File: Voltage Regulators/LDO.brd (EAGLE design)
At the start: 16.8 x 13.3 mm, 4 parts

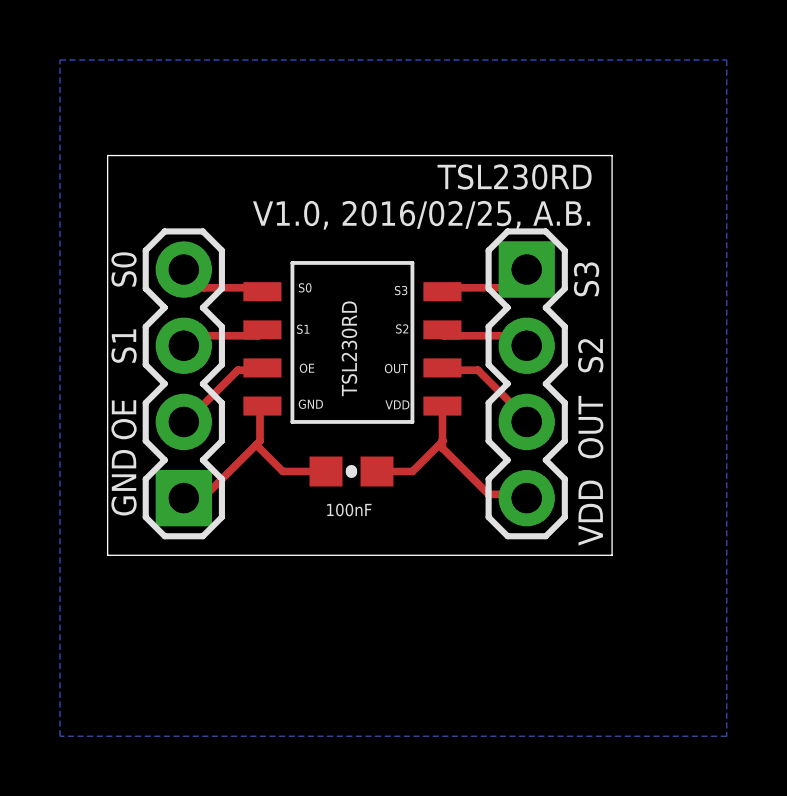
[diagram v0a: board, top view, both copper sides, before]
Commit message: new boards
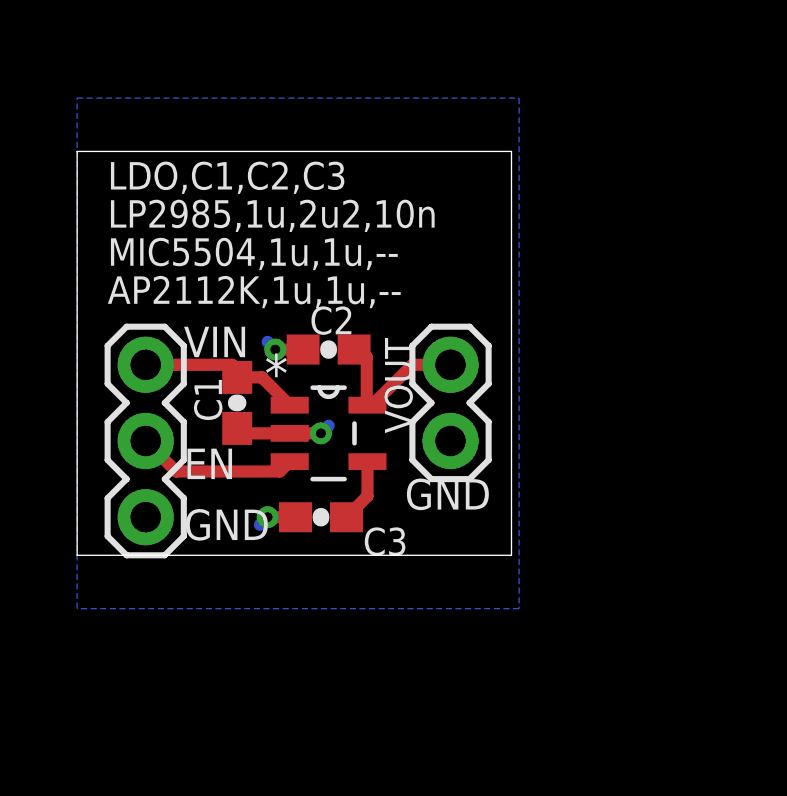
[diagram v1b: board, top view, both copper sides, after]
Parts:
- removed 100NF: 100nF, SparkFun-Capacitors:0603-CAP
- removed J1, J2: (no value), SparkFun-Connectors:1X04
- removed U$1: TSL230RDSMD, awqua_eagle_library:TSL230RD
- added C1, C2, C3: (no value), SparkFun-Passives:0603-CAP
- added FRAME1: FRAME-LETTER, SparkFun-Aesthetics:CREATIVE_COMMONS
- added JP1: (no value), SparkFun-Connectors:1X03
- added JP2: (no value), SparkFun-Connectors:1X02
- added U1: LP2985-33DBVT, LP2985-33DBVT:SOT95P280X145-5N
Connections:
- removed net N$1: J2.4, U$1.S0
- removed net N$2: J2.3, U$1.S1
- removed net N$3: J2.2, U$1.OE
- removed net N$5: J1.1, U$1.S3
- removed net N$6: J1.2, U$1.S2
- removed net N$7: J1.3, U$1.OUT
- removed net N$8: 100NF.1, J1.4, U$1.VDD
- new net BYPASS: C3.1, U1.4
- new net ENABLE: JP1.2, U1.3
- new net VIN: C1.1, JP1.3, U1.1
- new net VOUT: C2.1, JP2.1, U1.5
- net GND: now also C1.2, C2.2, C3.2, JP1.1, JP2.2, U1.2; no longer 100NF.2, J2.1, U$1.GND
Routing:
- net N$8: track 7.54 -> 0.00 mm
- net VIN: track 0.00 -> 5.47 mm
- net VOUT: track 0.00 -> 5.46 mm
- net ENABLE: track 0.00 -> 5.36 mm
- net N$7: track 3.62 -> 0.00 mm
- net N$3: track 3.34 -> 0.00 mm
- net N$5: track 3.22 -> 0.00 mm
- net N$6: track 3.15 -> 0.00 mm
- net N$1: track 2.91 -> 0.00 mm
- net N$2: track 2.85 -> 0.00 mm
- net BYPASS: track 0.00 -> 2.14 mm
- net GND: track 7.22 -> 6.09 mm, vias 0 -> 3
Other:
- board size 16.8 x 13.3 mm -> 14.5 x 13.5 mm
- board text added: "AP2112K,1u,1u,--"
- board text added: "EN"
- board text added: "LDO,C1,C2,C3"
- board text added: "LP2985,1u,2u2,10n"
- board text added: "MIC5504,1u,1u,--"
- board text added: "VIN"
- board text added: "VOUT"
- board text removed: "OE"
- board text removed: "OUT"
- board text removed: "S0"
- board text removed: "S1"
- board text removed: "S2"
- board text removed: "S3"
- board text removed: "TSL230RD V1.0, 2016/02/25, A.B."
- board text removed: "VDD"
